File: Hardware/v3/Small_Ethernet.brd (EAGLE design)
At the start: 64.5 x 33.4 mm, 51 parts, among them U1 EDISON_CONNECTOR_FULLMOUNTING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, U2 LAN9512-JZX, U3 MAX4995AAUT+, U4 EDISON_CONNECTOR_FULLHEADER, X1 J1011F01P

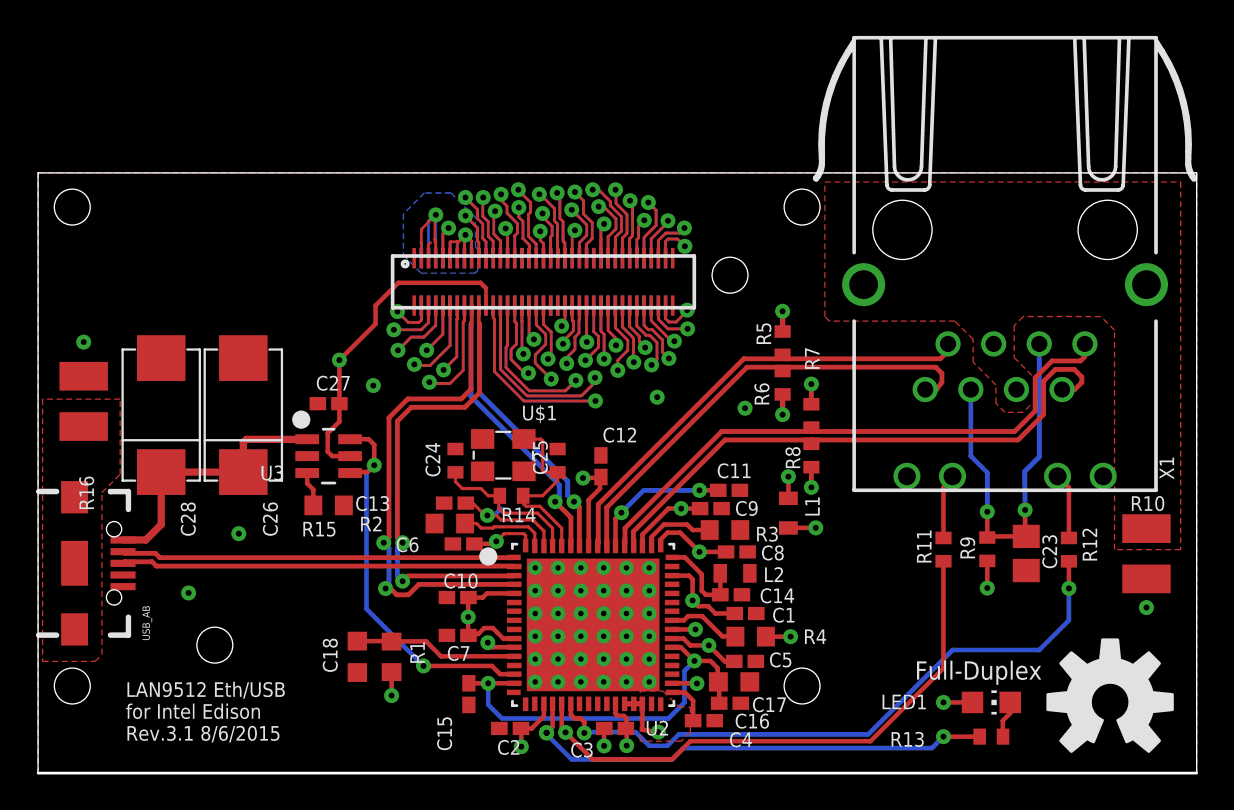
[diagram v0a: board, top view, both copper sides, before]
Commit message: Ready for final review
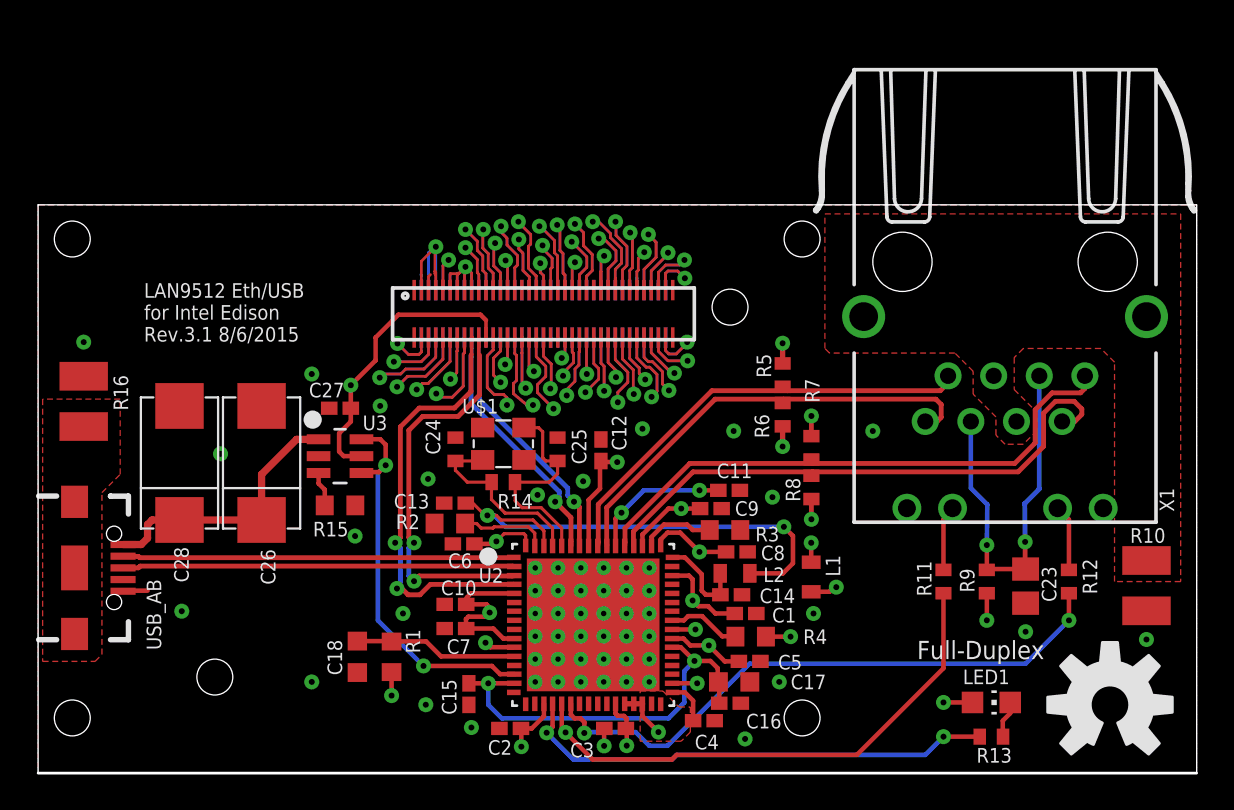
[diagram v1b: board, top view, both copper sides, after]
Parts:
- moved L1 3.78 mm to (43.1, 10.9)
- moved C26 2.85 mm to (12.4, 17.3)
- moved C28 2.85 mm to (7.87, 17.3)
- moved C23 1.82 mm to (55.0, 10.4)
- moved R9 1.80 mm to (52.8, 10.7)
- moved R6 1.78 mm to (41.5, 20.0)
- moved U1 1.78 mm to (40.5, 28.9)
- moved R10 1.78 mm to (61.7, 10.4)
- moved R11 1.78 mm to (50.4, 10.7)
- moved R12 1.78 mm to (57.4, 10.7)
- moved R8 1.78 mm to (43.1, 15.9)
- moved R5 1.78 mm to (41.5, 22.2)
- moved R7 1.78 mm to (43.1, 18.1)
- moved U4 1.78 mm to (28.1, 25.6)
- moved X1 1.78 mm to (53.8, 22.1)
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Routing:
- net N$1: track 6.75 -> 27.5 mm, vias 1 -> 2
- net P24: track 20.0 -> 5.62 mm
- net P26: track 16.3 -> 3.11 mm
- net P22: track 20.0 -> 9.33 mm
- net USB_D_P: track 27.4 -> 24.1 mm
- net USB_D_N: track 25.7 -> 22.4 mm
- net P12: track 7.80 -> 4.94 mm
- net VDD33A: track 52.9 -> 55.5 mm
- net P14: track 11.7 -> 9.17 mm
- net USB_VBUS: track 18.4 -> 16.3 mm
- net N$21: track 8.48 -> 10.4 mm
- net P6: track 7.56 -> 9.38 mm
- net USBUP_P: track 16.0 -> 14.2 mm
- net N$18: track 35.6 -> 33.9 mm
- net USBUP_N: track 15.7 -> 14.0 mm
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- added copper zone on layer 3, net GND
- removed copper zone on layer 3, net USB_REF
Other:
- board size 64.5 x 33.4 mm -> 64.5 x 31.6 mm
